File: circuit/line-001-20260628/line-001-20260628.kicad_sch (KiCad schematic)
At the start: 220 parts, among them J1 Conn_01x02_Pin, J2 Conn_01x02_Pin, J3 Conn_02x03_Odd_Even, J4 USB_C_Receptacle_USB2.0_16P, Q1 Q_Photo_NPN_CE, Q10 Q_Photo_NPN_CE, Q11 Q_Photo_NPN_CE, Q12 Q_Photo_NPN_CE, Q13 Q_Photo_NPN_CE, Q14 Q_Photo_NPN_CE, Q15 Q_Photo_NPN_CE, Q16 Q_Photo_NPN_CE, Q17 Q_Photo_NPN_CE, Q18 Q_Photo_NPN_CE, Q19 Q_Photo_NPN_CE, Q2 Q_Photo_NPN_CE, Q20 Q_Photo_NPN_CE, Q21 Q_Photo_NPN_CE, Q22 Q_Photo_NPN_CE, Q23 Q_Photo_NPN_CE, Q24 Q_Photo_NPN_CE, Q25 Q_Photo_NPN_CE, Q26 Q_Photo_NPN_CE, Q27 Q_Photo_NPN_CE, Q28 Q_Photo_NPN_CE, Q29 Q_Photo_NPN_CE, Q3 Q_Photo_NPN_CE, Q30 Q_Photo_NPN_CE, Q31 Q_Photo_NPN_CE, Q32 Q_Photo_NPN_CE, Q37 Q_Photo_NPN_CE, Q38 Q_Photo_NPN_CE, Q39 Q_Photo_NPN_CE, Q4 Q_Photo_NPN_CE, Q40 Q_Photo_NPN_CE, Q5 Q_Photo_NPN_CE, Q6 Q_Photo_NPN_CE, Q7 Q_Photo_NPN_CE, Q8 Q_Photo_NPN_CE, Q9 Q_Photo_NPN_CE, SW1 SW_Push, SW2 SW_SPDT, U1 LM393DR, U10 LM393DR, U11 LM393DR, U12 LM393DR, U13 LM393DR, U14 LM393DR, U15 LM393DR, U16 LM393DR, U17 ATmega2560-16A, U18 CH340G, U2 LM393DR, U3 LM393DR, U4 LM393DR, U5 LM393DR, U6 LM393DR, U7 LM393DR, U8 LM393DR, U9 LM393DR, Y1 16MHz, Y2 12MHz

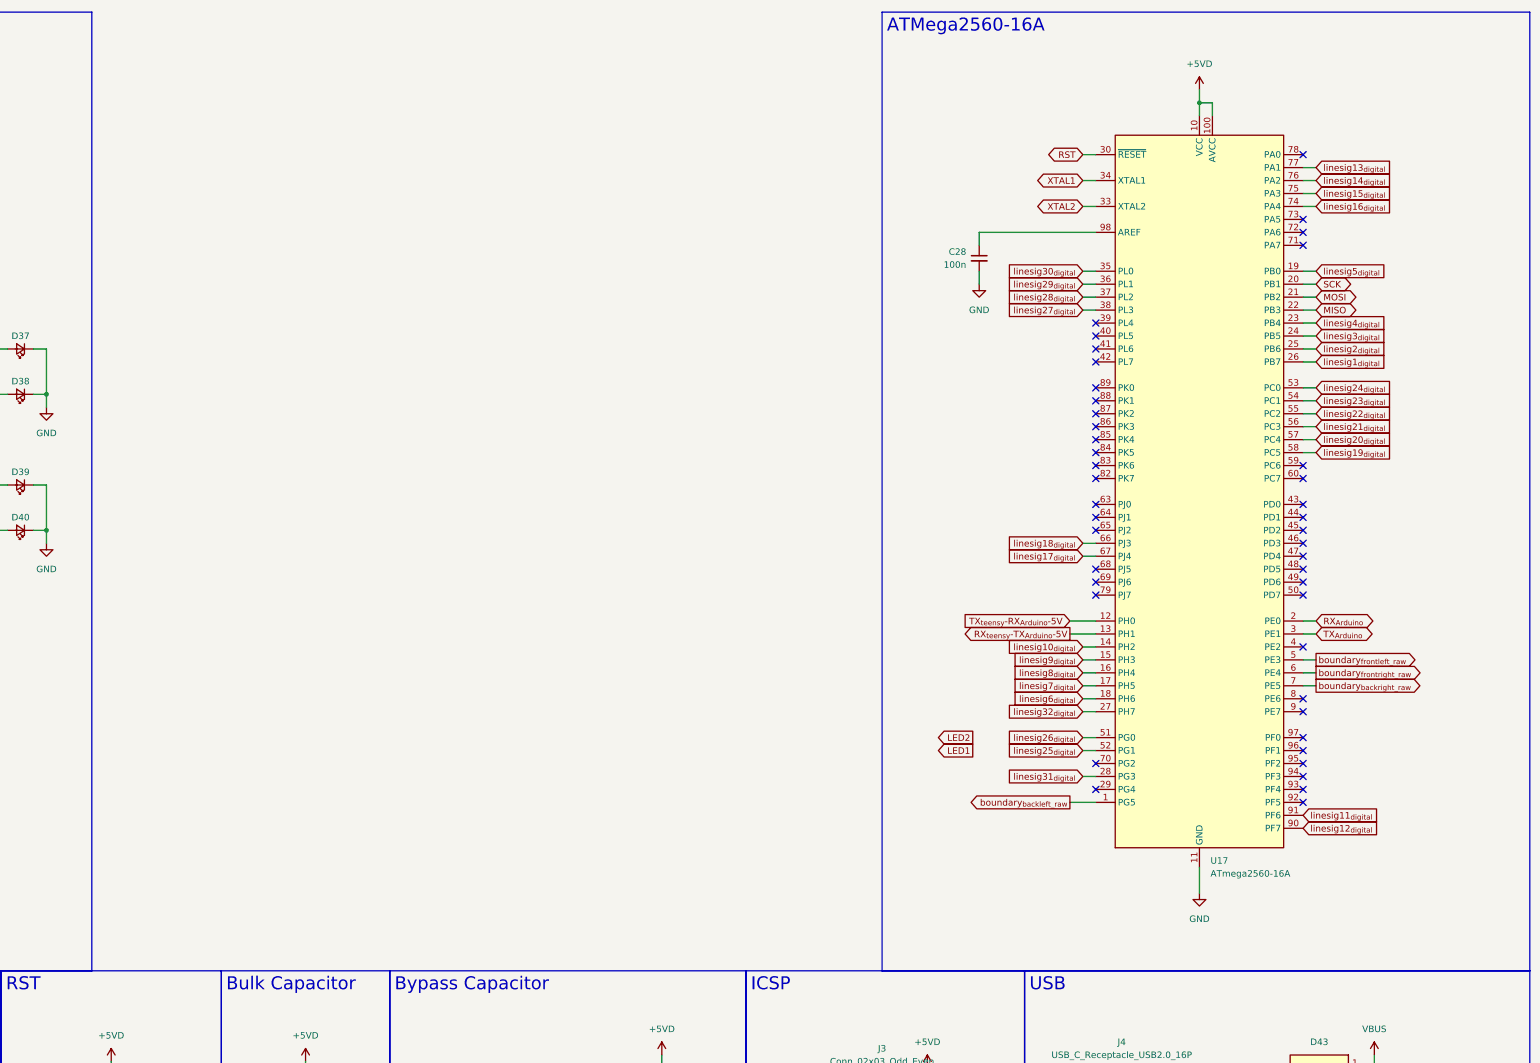
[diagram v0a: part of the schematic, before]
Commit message: Update ラインセンサ基板のPCBを進めた
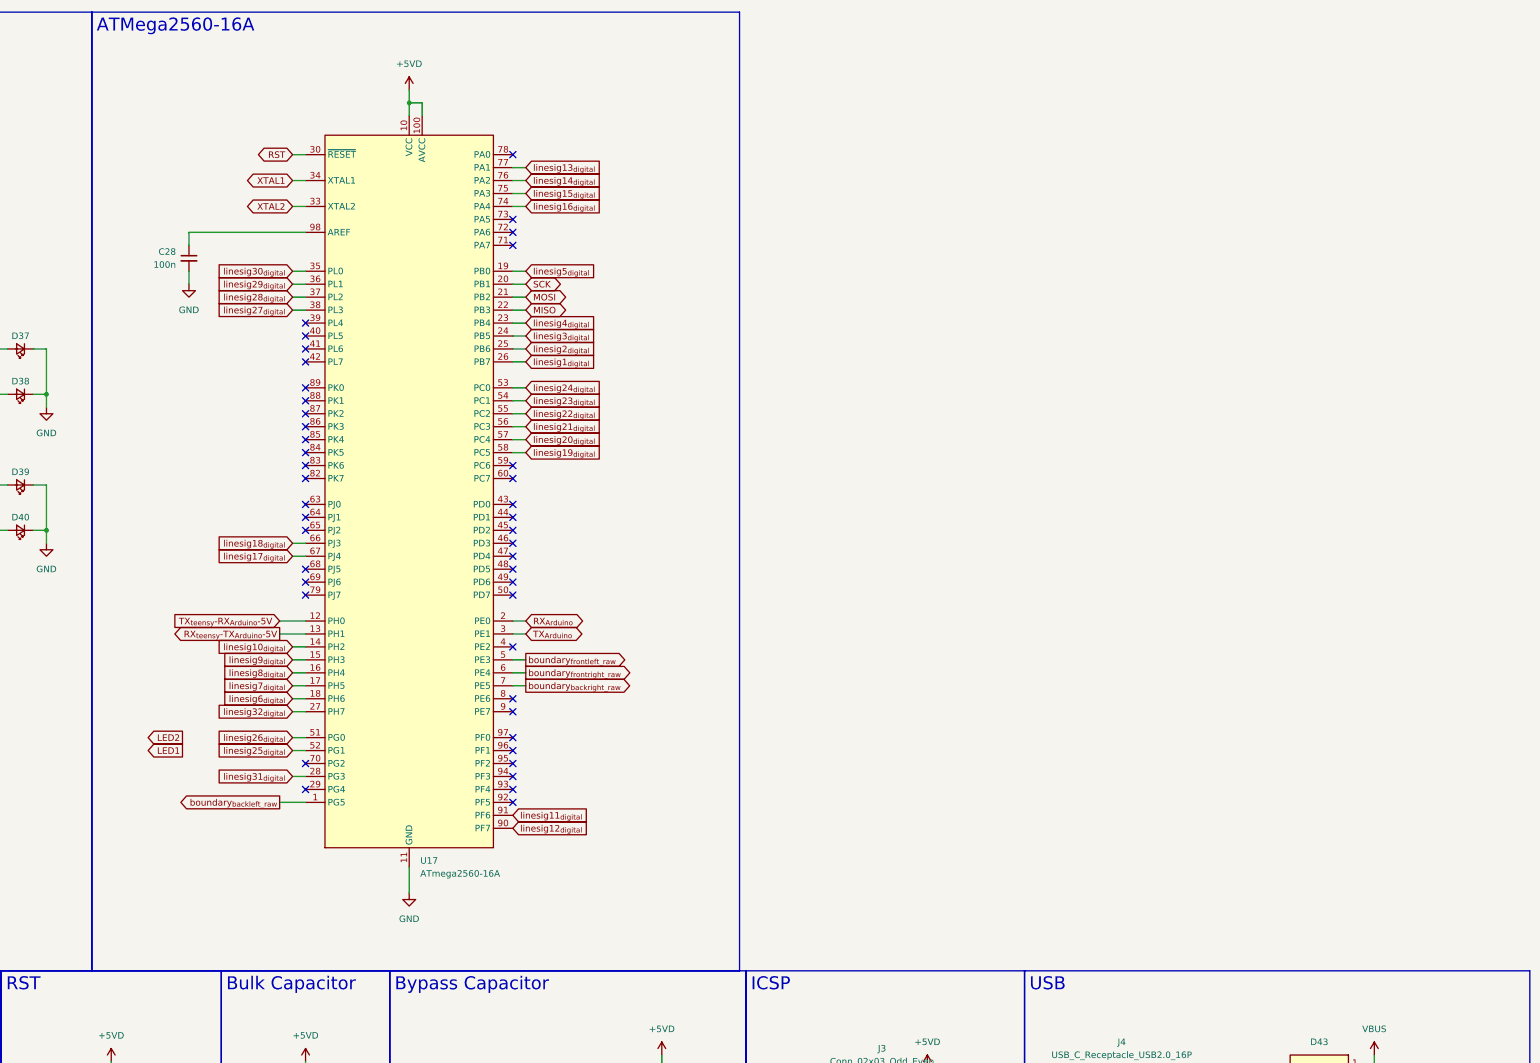
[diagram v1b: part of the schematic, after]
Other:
- moved on the sheet: C28, U17
